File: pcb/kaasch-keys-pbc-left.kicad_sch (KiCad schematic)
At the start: 73 parts, among them J1 Conn_01x12_Pin, J2 Conn_01x12_Pin, SW1 SW_Push, SW10 SW_Push, SW11 SW_Push, SW12 SW_Push, SW13 SW_Push, SW14 SW_Push, SW15 SW_Push, SW16 SW_Push, SW17 SW_Push, SW18 SW_Push, SW19 SW_Push, SW2 SW_Push, SW20 SW_Push, SW21 SW_Push, SW22 SW_Push, SW23 SW_Push, SW24 SW_Push, SW25 SW_Push, SW26 SW_Push, SW27 SW_Push, SW28 SW_Push, SW29 SW_Push, SW3 SW_Push, SW30 SW_Push, SW31 SW_Push, SW32 SW_Push, SW33 SW_Push, SW34 SW_Push, SW35 SW_Push, SW36 SW_Push_Reset, SW4 SW_Push, SW5 SW_Push, SW6 SW_Push, SW7 SW_Push, SW8 SW_Push, SW9 SW_Push

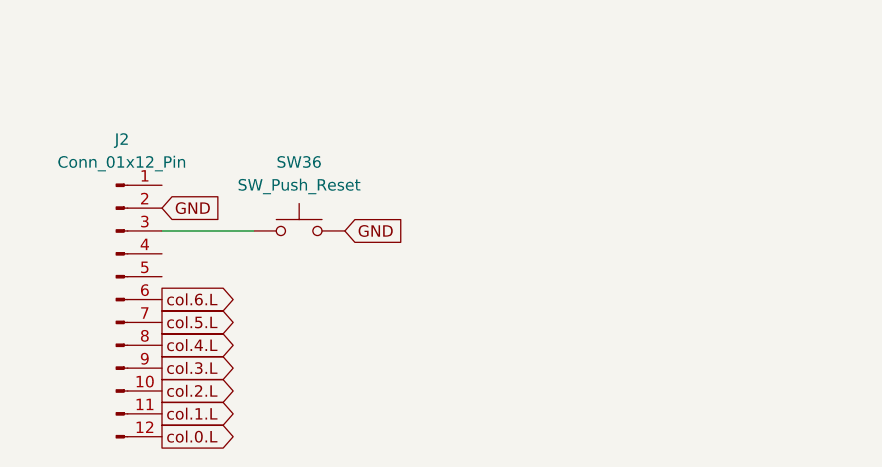
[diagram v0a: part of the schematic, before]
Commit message: continue on design
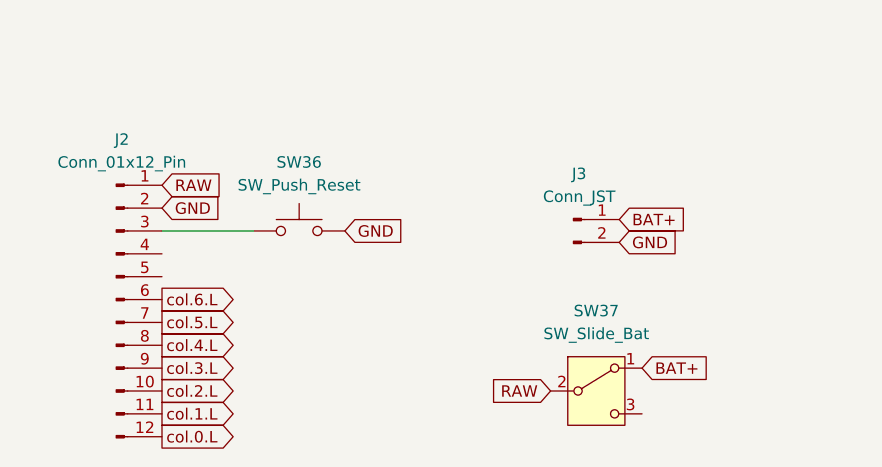
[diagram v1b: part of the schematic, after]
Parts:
- added J3: Conn_JST, Connector_JST:JST_EH_B2B-EH-A_1x02_P2.50mm_Vertical, symbol Connector:Conn_01x02_Pin
- added SW37: SW_Slide_Bat, Button_Switch_SMD:SW_SPDT_PCM12, symbol Switch:SW_SPDT
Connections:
- net GND: now also J3.2 (Pin_2)
- net RAW: now reaches J2.1 (Pin_1)
- net RAW: now also SW37.2 (B)
- new net BAT+: J3.1 (Pin_1), SW37.1 (A)
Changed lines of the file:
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@@
 		)
 	)
+	(global_label "BAT+"
+		(shape input)
+		(at 148.59 172.72 0)
+		(fields_autoplaced yes)
+		(effects
+			(font
+				(size 1.27 1.27)
+			)
+			(justify left)
+		)
+		(property "Intersheetrefs" "${INTERSHEET_REFS}"
+			(at 156.4738 172.72 0)
+			(effects
+				(font
+					(size 1.27 1.27)
+				)
+				(justify left)
+				(hide yes)
+			)
+		)
+	)
 	(global_label "row.0.L"
 		(shape input)
@@
 		)
 	)
+	(global_label "RAW"
+		(shape input)
+		(at 138.43 175.26 180)
+		(fields_autoplaced yes)
+		(effects
+			(font
+				(size 1.27 1.27)
+			)
+			(justify right)
+		)
+		(property "Intersheetrefs" "${INTERSHEET_REFS}"
+			(at 131.6348 175.26 0)
+			(effects
+				(font
+					(size 1.27 1.27)
+				)
+				(justify right)
+				(hide yes)
+			)
+		)
+	)
 	(global_label "GND"
 		(shape input)
@@
 		)
 	)
+	(global_label "RAW"
+		(shape input)
+		(at 95.25 152.4 0)
+		(fields_autoplaced yes)
+		(effects
+			(font
+				(size 1.27 1.27)
+			)
+			(justify left)
+		)
+		(property "Intersheetrefs" "${INTERSHEET_REFS}"
+			(at 102.0452 152.4 0)
+			(effects
+				(font
+					(size 1.27 1.27)
+				)
+				(justify left)
+				(hide yes)
+			)
+		)
+	)
 	(global_label "col.1.L"
 		(shape output)
@@
 		)
 	)
+	(global_label "GND"
+		(shape input)
+		(at 146.05 158.75 0)
+		(fields_autoplaced yes)
+		(effects
+			(font
+				(size 1.27 1.27)
+			)
+			(justify left)
+		)
+		(property "Intersheetrefs" "${INTERSHEET_REFS}"
+			(at 152.9057 158.75 0)
+			(effects
+				(font
+					(size 1.27 1.27)
+				)
+				(justify left)
+				(hide yes)
+			)
+		)
+	)
 	(global_label "row.4.L"
 		(shape output)
@@
 		)
 	)
+	(global_label "BAT+"
+		(shape input)
+		(at 146.05 156.21 0)
+		(fields_autoplaced yes)
+		(effects
+			(font
+				(size 1.27 1.27)
+			)
+			(justify left)
+		)
+		(property "Intersheetrefs" "${INTERSHEET_REFS}"
+			(at 153.9338 156.21 0)
+			(effects
+				(font
+					(size 1.27 1.27)
+				)
+				(justify left)
+				(hide yes)
+			)
+		)
+	)
 	(global_label "col.6.L"
 		(shape input)
@@
 	)
 	(symbol
+		(lib_id "Switch:SW_SPDT")
+		(at 143.51 175.26 0)
+		(unit 1)
+		(exclude_from_sim no)
+		(in_bom yes)
+		(on_board yes)
+		(dnp no)
+		(fields_autoplaced yes)
+		(property "Reference" "SW37"
+			(at 143.51 166.37 0)
+			(effects
+				(font
+					(size 1.27 1.27)
+				)
+			)
+		)
+		(property "Value" "SW_Slide_Bat"
+			(at 143.51 168.91 0)
+			(effects
+				(font
+					(size 1.27 1.27)
+				)
+			)
+		)
+		(property "Footprint" "Button_Switch_SMD:SW_SPDT_PCM12"
+			(at 143.51 175.26 0)
+			(effects
+				(font
+					(size 1.27 1.27)
+				)
+				(hide yes)
+			)
+		)
+		(property "Datasheet" "~"
+			(at 143.51 182.88 0)
+			(effects
+				(font
+					(size 1.27 1.27)
+				)
+				(hide yes)
+			)
+		)
+		(property "Description" "Switch, single pole double throw"
+			(at 143.51 175.26 0)
+			(effects
+				(font
+					(size 1.27 1.27)
+				)
+				(hide yes)
+			)
+		)
+		(pin "1"
+		)
+		(pin "3"
+		)
+		(pin "2"
+		)
+		(instances
+			(project ""
+				(path "/71cf87fc-58ce-4acc-b054-5cde32e406ee"
+					(reference "SW37")
+					(unit 1)
+				)
+			)
+		)
+	)
+	(symbol
 		(lib_id "Diode:1N4148")
 		(at 176.53 109.22 90)
@@
 					(unit 1)
 				)
+			)
+		)
+	)
+	(symbol
+		(lib_id "Connector:Conn_01x02_Pin")
+		(at 140.97 156.21 0)
+		(unit 1)
+		(exclude_from_sim no)
+		(in_bom yes)
+		(on_board yes)
+		(dnp no)
+		(fields_autoplaced yes)
+		(property "Reference" "J3"
+			(at 141.605 151.13 0)
+			(effects
+				(font
+					(size 1.27 1.27)
+				)
+			)
+		)
+		(property "Value" "Conn_JST"
+			(at 141.605 153.67 0)
+			(effects
+				(font
+					(size 1.27 1.27)
+				)
+			)
+		)
+		(property "Footprint" "Connector_JST:JST_EH_B2B-EH-A_1x02_P2.50mm_Vertical"
+			(at 140.97 156.21 0)
+			(effects
+				(font
+					(size 1.27 1.27)
+				)
+				(hide yes)
+			)
+		)
+		(property "Datasheet" "~"
+			(at 140.97 156.21 0)
+			(effects
+				(font
+					(size 1.27 1.27)
+				)
+				(hide yes)
+			)
+		)
+		(property "Description" "Generic connector, single row, 01x02, script generated"
+			(at 140.97 156.21 0)
+			(effects
+				(font
+					(size 1.27 1.27)
+				)
+				(hide yes)
+			)
+		)
+		(pin "1"
+		)
+		(pin "2"
+		)
+		(instances
+			(project ""
+				(path "/71cf87fc-58ce-4acc-b054-5cde32e406ee"
+					(reference "J3")
+					(unit 1)
+				)
